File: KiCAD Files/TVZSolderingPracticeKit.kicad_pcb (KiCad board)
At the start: 2 copper layers, 12 parts, among them SW10 SW_SPDT, U1 NE555P

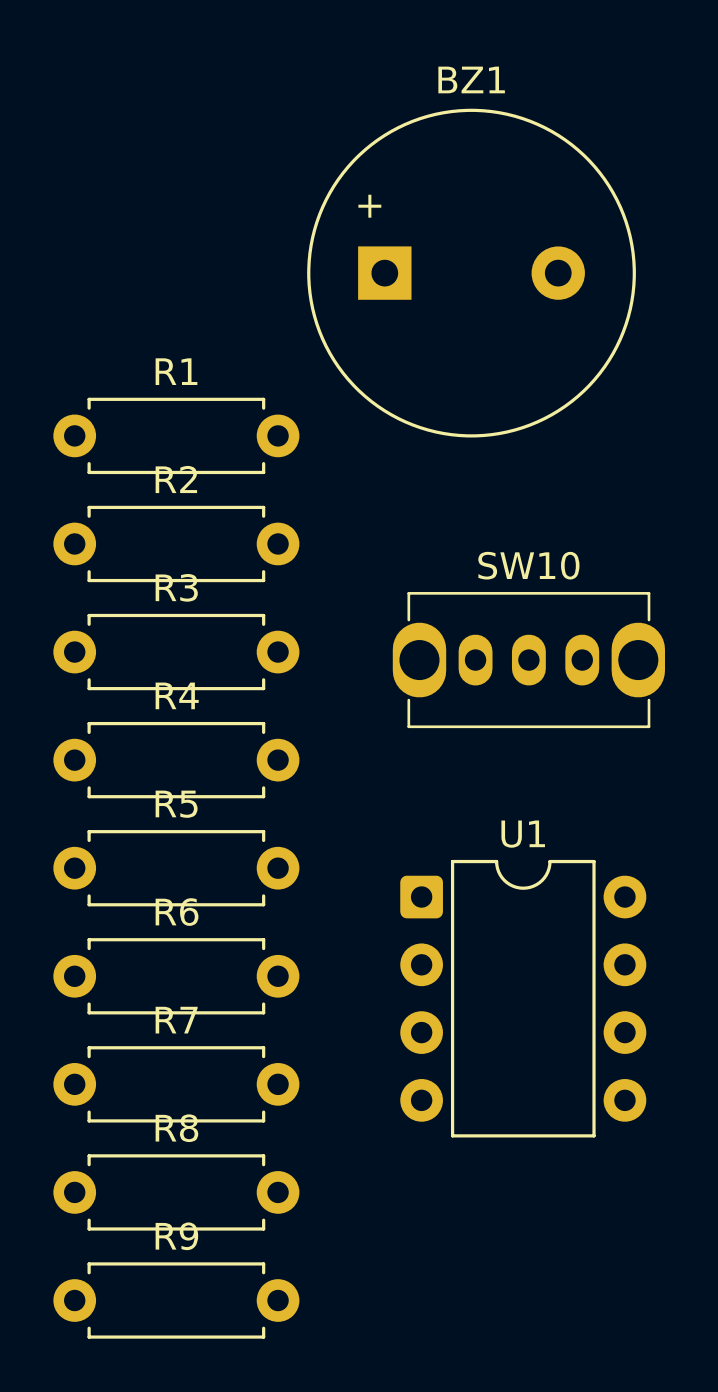
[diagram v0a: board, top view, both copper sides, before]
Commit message: update
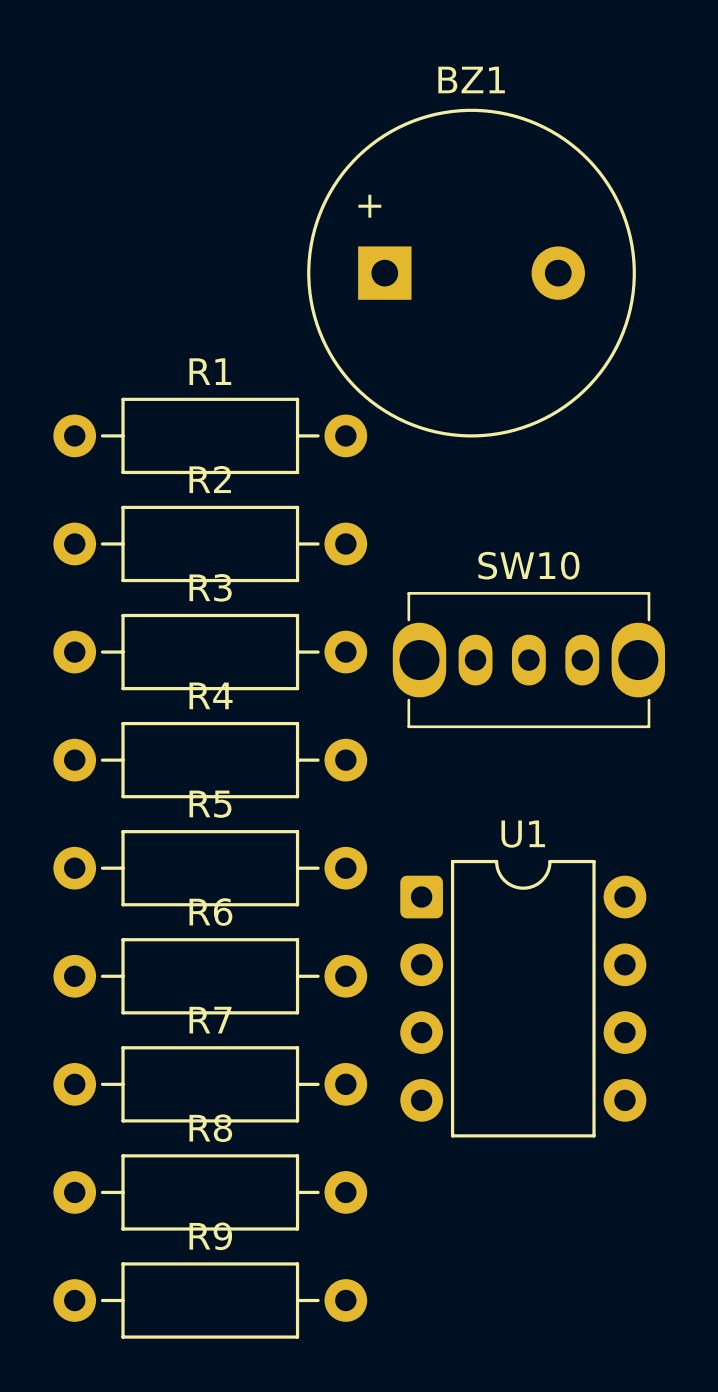
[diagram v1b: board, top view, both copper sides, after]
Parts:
- R1, R2, R3, R4, R5, R6, R7, R8, R9: footprint Resistor_THT:R_Axial_DIN0207_L6.3mm_D2.5mm_P7.62mm_Horizontal -> Resistor_THT:R_Axial_DIN0207_L6.3mm_D2.5mm_P10.16mm_Horizontal
